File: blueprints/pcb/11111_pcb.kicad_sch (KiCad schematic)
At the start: 132 parts, among them J1 TRRS_MJ-4PP-9, J2 TRRS_MJ-4PP-9, SW1 SW_Push, SW10 SW_Push, SW11 SW_Push, SW12 SW_Push, SW13 SW_Push, SW14 SW_Push, SW15 SW_Push, SW16 SW_Push, SW17 SW_Push, SW18 SW_Push, SW19 SW_Push, SW2 SW_Push, SW20 SW_Push, SW21 SW_Push, SW22 SW_Push, SW23 SW_Push, SW24 SW_Push, SW25 SW_Push, SW26 SW_Push, SW27 SW_Push, SW28 SW_Push, SW29 SW_Push, SW3 SW_Push, SW30 SW_Push, SW31 SW_Push, SW32 SW_Push, SW33 SW_Push, SW34 SW_Push, SW35 SW_Push, SW36 SW_Push, SW37 SW_Push, SW38 SW_Push, SW39 SW_Push, SW4 SW_Push, SW40 SW_Push, SW41 SW_Push, SW42 SW_Push, SW43 SW_Push, SW44 SW_Push, SW45 SW_Push, SW46 SW_Push, SW47 SW_Push, SW48 SW_Push, SW49 SW_Push, SW5 SW_Push, SW50 SW_Push, SW51 SW_Push, SW52 SW_Push, SW53 SW_Push, SW54 SW_Push, SW55 SW_Push, SW56 SW_Push, SW57 SW_Push, SW58 SW_Push, SW59 SW_Push, SW6 SW_Push, SW60 SW_Push, SW61 SW_Push, SW62 SW_Push, SW63 SW_Push, SW64 SW_Push, SW7 SW_Push, SW8 SW_Push, SW9 SW_Push, U1 Pico, U2 Pico

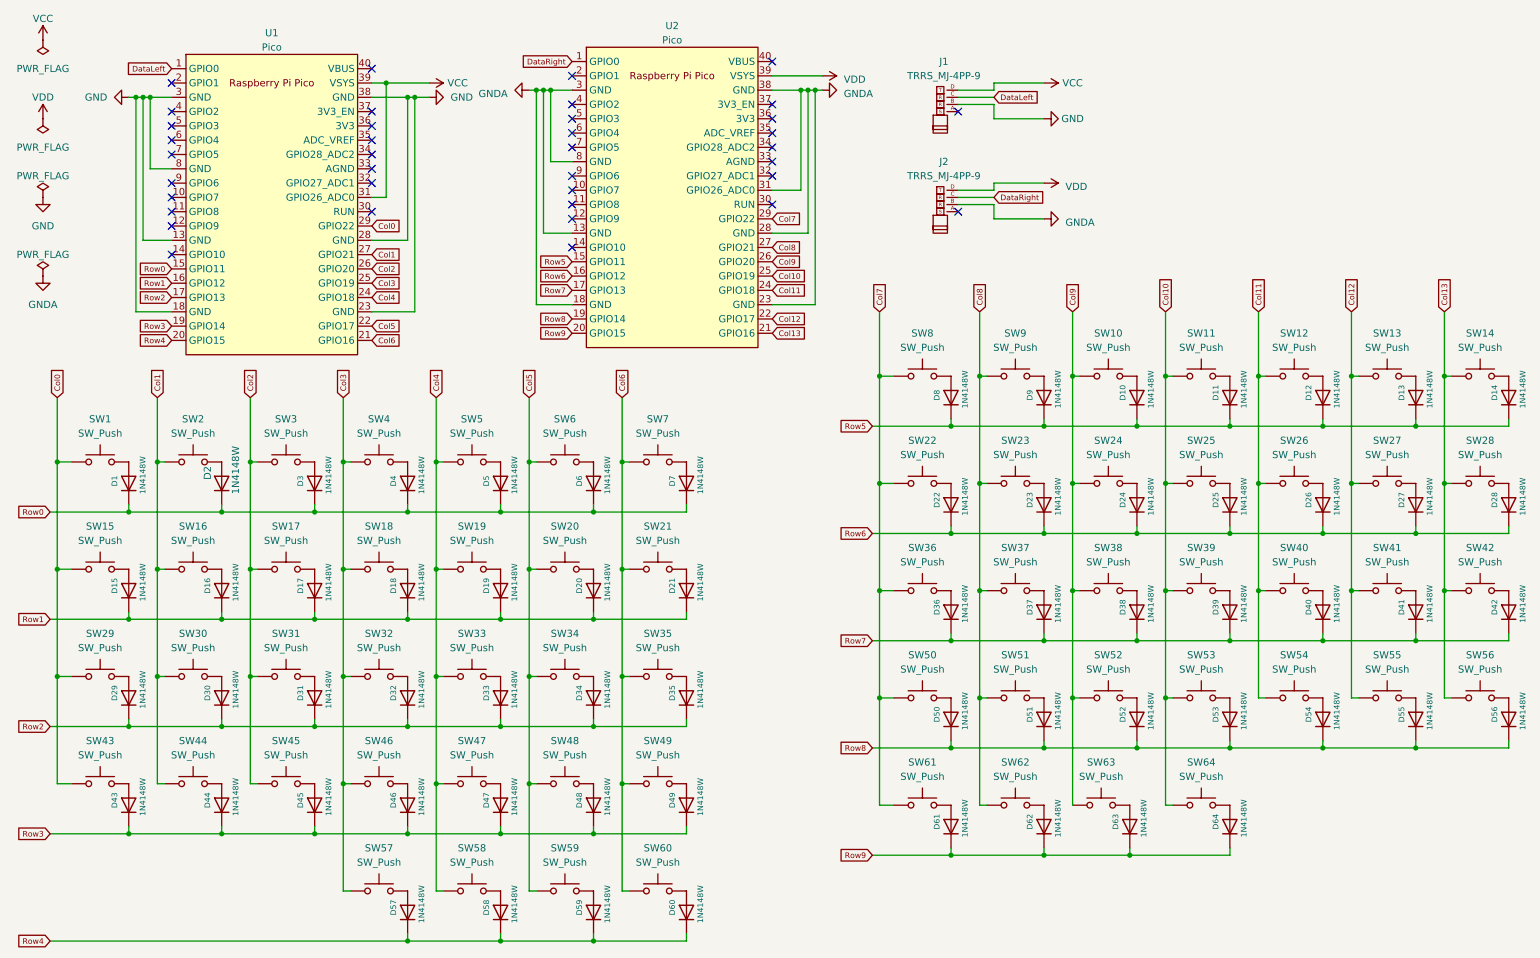
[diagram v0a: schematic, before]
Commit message: version3
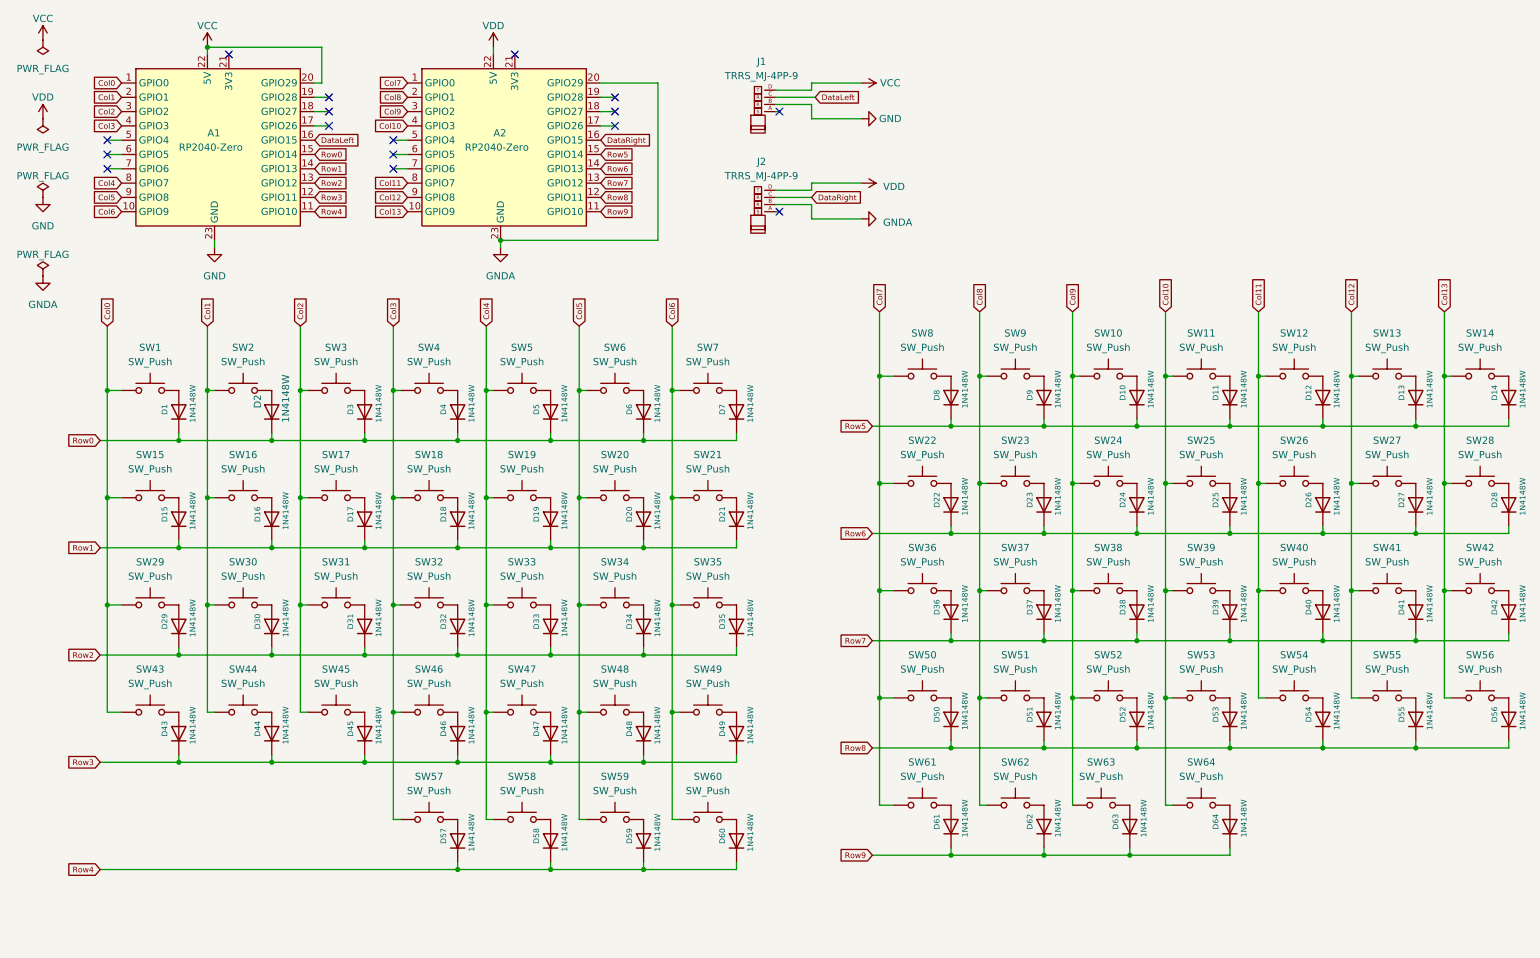
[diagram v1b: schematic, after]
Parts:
- removed U1, U2: Pico, Raspberry-pi-pico:RPi_Pico_SMD_TH, symbol raspberry-pi-pico:Pico
- added A1, A2: RP2040-Zero, RP2040-zero:RP2040-Zero_through_hole_omit, symbol RP2040-zero:RP2040-Zero
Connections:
- net Col0: now also A1.1 (GPIO0)
- net Col1: now also A1.2 (GPIO1)
- net Col10: now also A2.4 (GPIO3)
- net Col11: now also A2.8 (GPIO7)
- net Col12: now also A2.9 (GPIO8)
- net Col13: now also A2.10 (GPIO9)
- net Col2: now also A1.3 (GPIO2)
- net Col3: now also A1.4 (GPIO3)
- net Col4: now also A1.8 (GPIO7)
- net Col5: now also A1.9 (GPIO8)
- net Col6: now also A1.10 (GPIO9)
- net Col7: now also A2.1 (GPIO0)
- net Col8: now also A2.2 (GPIO1)
- net Col9: now also A2.3 (GPIO2)
- net DataLeft: now also A1.16 (GPIO15)
- net DataRight: now also A2.16 (GPIO15)
- net GND: now also A1.23 (GND)
- net GNDA: now also A2.20 (GPIO29), A2.23 (GND)
- net Row0: now also A1.15 (GPIO14)
- net Row1: now also A1.14 (GPIO13)
- net Row2: now also A1.13 (GPIO12)
- net Row3: now also A1.12 (GPIO11)
- net Row4: now also A1.11 (GPIO10)
- net Row5: now also A2.15 (GPIO14)
- net Row6: now also A2.14 (GPIO13)
- net Row7: now also A2.13 (GPIO12)
- net Row8: now also A2.12 (GPIO11)
- net Row9: now also A2.11 (GPIO10)
- net VCC: now also A1.20 (GPIO29), A1.22 (5V)
- net VDD: now also A2.22 (5V)
- no-connect marks 38 -> 16
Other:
- moved on the sheet: D1, D15, D16, D17, D18, D19, D2, D20, D21, D29, D3, D30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
